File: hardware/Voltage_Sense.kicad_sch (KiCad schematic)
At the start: 56 parts, among them U5 TLV9002QDRQ1, U6 AMC3311QDWERQ1, U7 AMC3311QDWERQ1

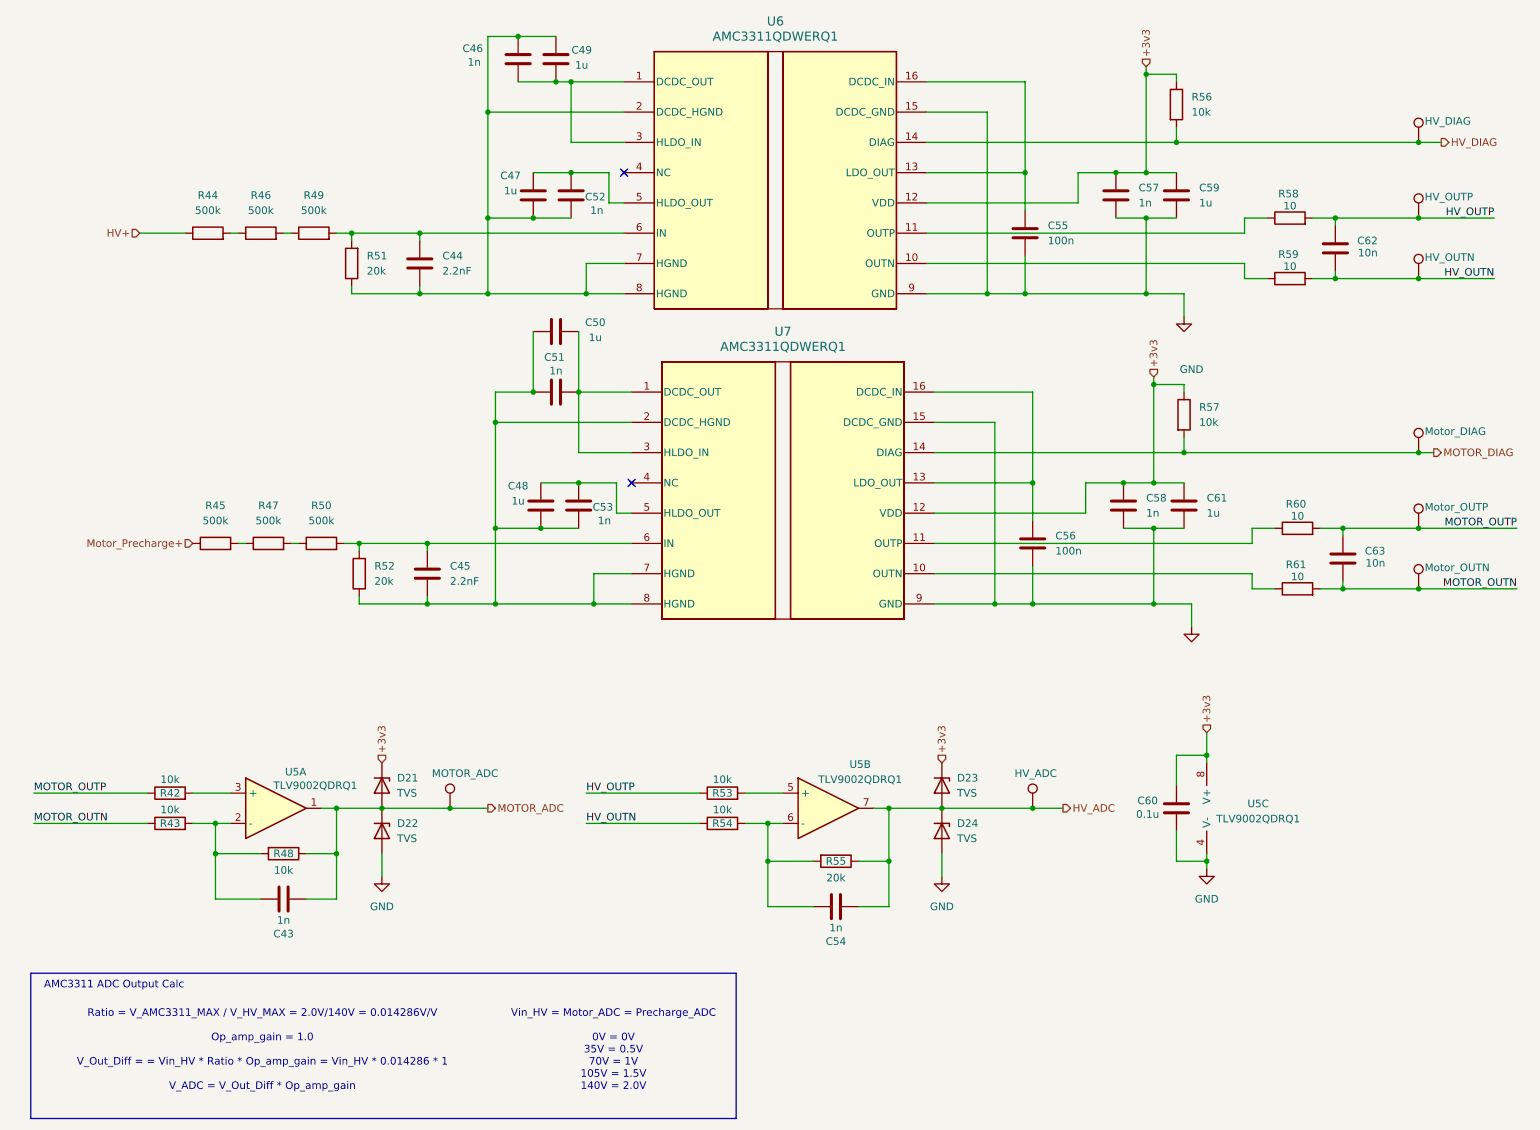
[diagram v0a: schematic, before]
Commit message: added 1% calcs
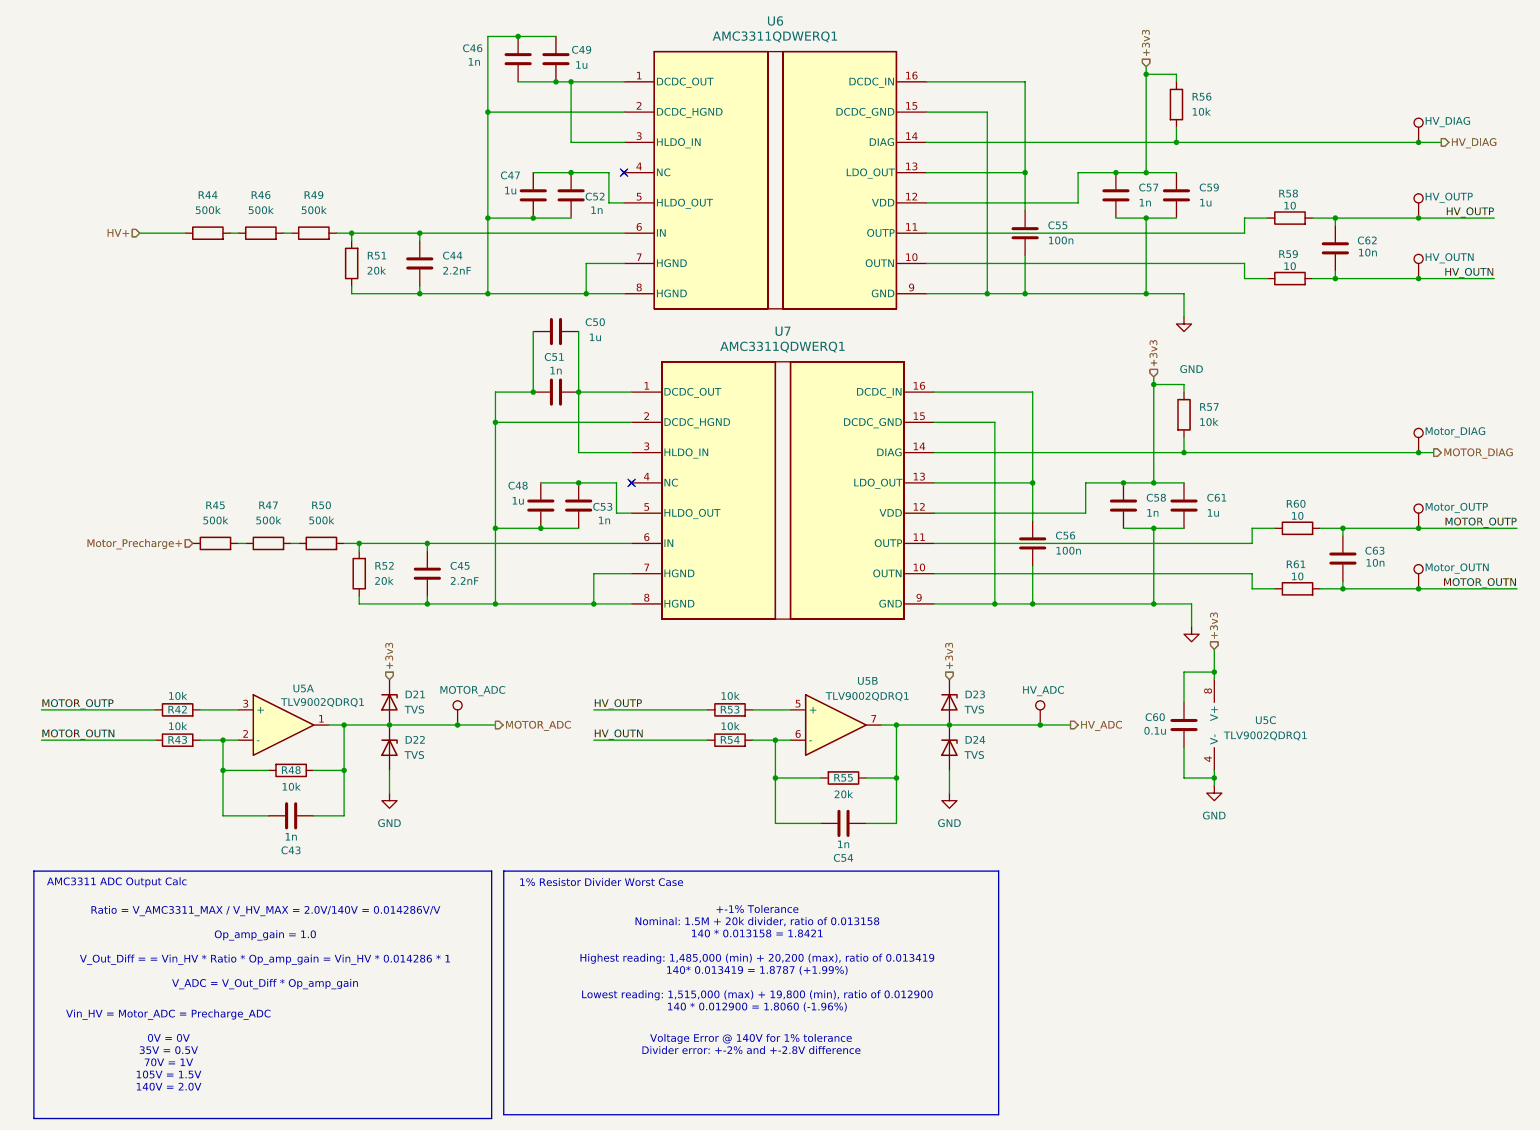
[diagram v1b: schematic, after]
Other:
- note added: "+-1% Tolerance Nominal: 1.5M + 20k divider, ratio of 0.013158 140 * 0.013158 = 1.8421 Highest reading: 1,485,000 (min) + 20,200 (max), ratio of 0.013419 140* 0.013419 = 1.8787 (+1.99%) Lowest reading: 1,515,000 (max) + 19,800 (min), ratio of 0.012900 140 * 0.012900 = 1.8060 (-1.96%)"
- note added: "1% Resistor Divider Worst Case"
- note added: "Voltage Error @ 140V for 1% tolerance Divider error: +-2% and +-2.8V difference"
- moved on the sheet: C43, C54, C60, D21, D22, D23, D24, R42, R43, R48, R53, R54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
